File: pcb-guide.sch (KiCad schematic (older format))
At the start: 14 parts

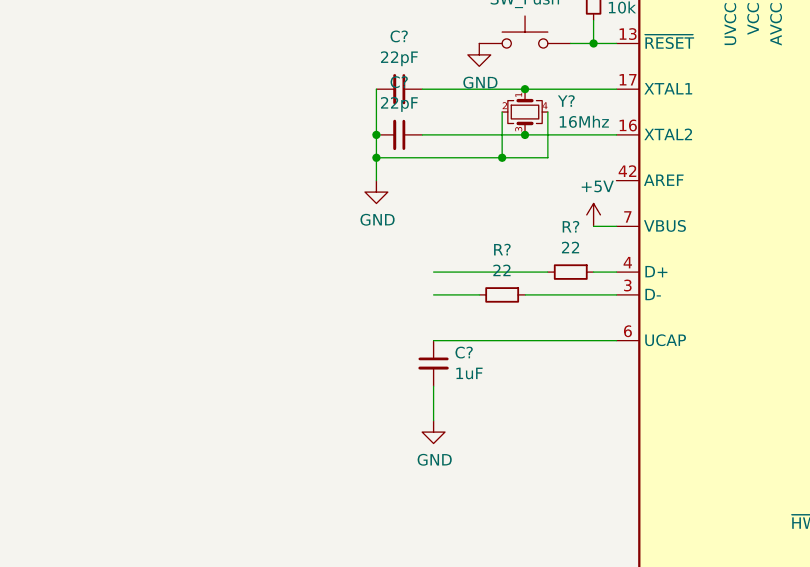
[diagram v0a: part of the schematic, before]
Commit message: Tags added
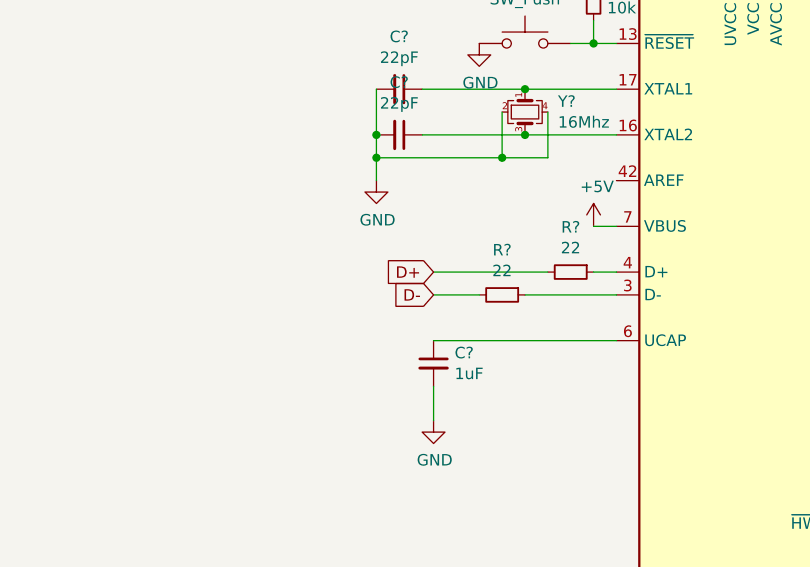
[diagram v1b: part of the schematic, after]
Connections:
- net labels added: D+, D-
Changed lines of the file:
@@
 Wire Wire Line
 	2250 1400 2350 1400
+Text GLabel 1550 2400 0    50   Input ~ 0
+D+
+Text GLabel 1550 2500 0    50   Input ~ 0
+D-
 $EndSCHEMATC
